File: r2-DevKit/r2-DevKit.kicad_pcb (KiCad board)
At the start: 4 copper layers, 92.3 x 67.1 mm, 33 parts, among them CON1 USB-MICRO-B, J1 CONN_01X05, J10 Battery SW, J11 OPTS, J2 CONN_01X08, J3 CONN_01X14, J4 CONN_01X02, J5 CONN_01X08, J6 CONN_01X14, J7 Li-Po, J8 JTAG, J9 CONN_02X15, P1 Compute Socket, P2 Sensor Socket, P3 CONN_01X01, P4 CONN_01X01, SW3 Pin_0, SW4 CHIP_PU, U1 EMIF02-USB03F2

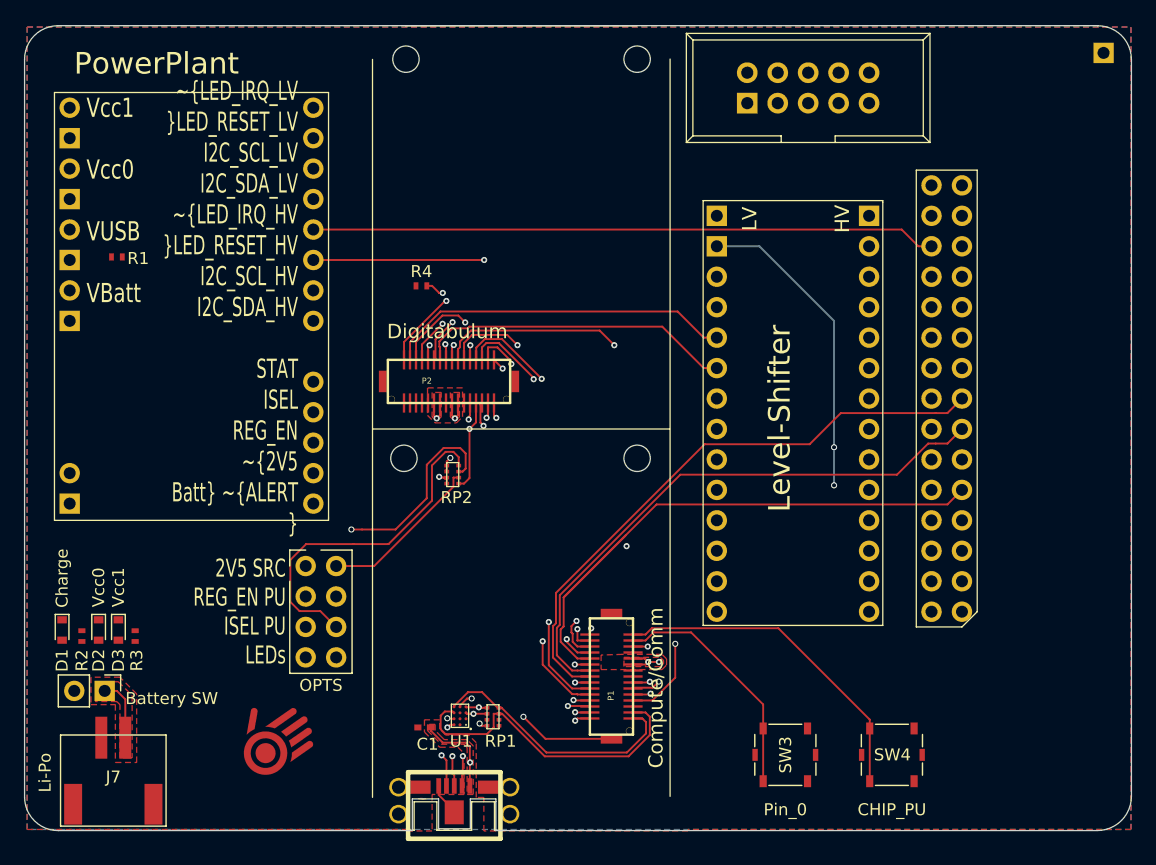
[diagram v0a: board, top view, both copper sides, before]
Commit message: Fixed some bugs in the Dev Harness.
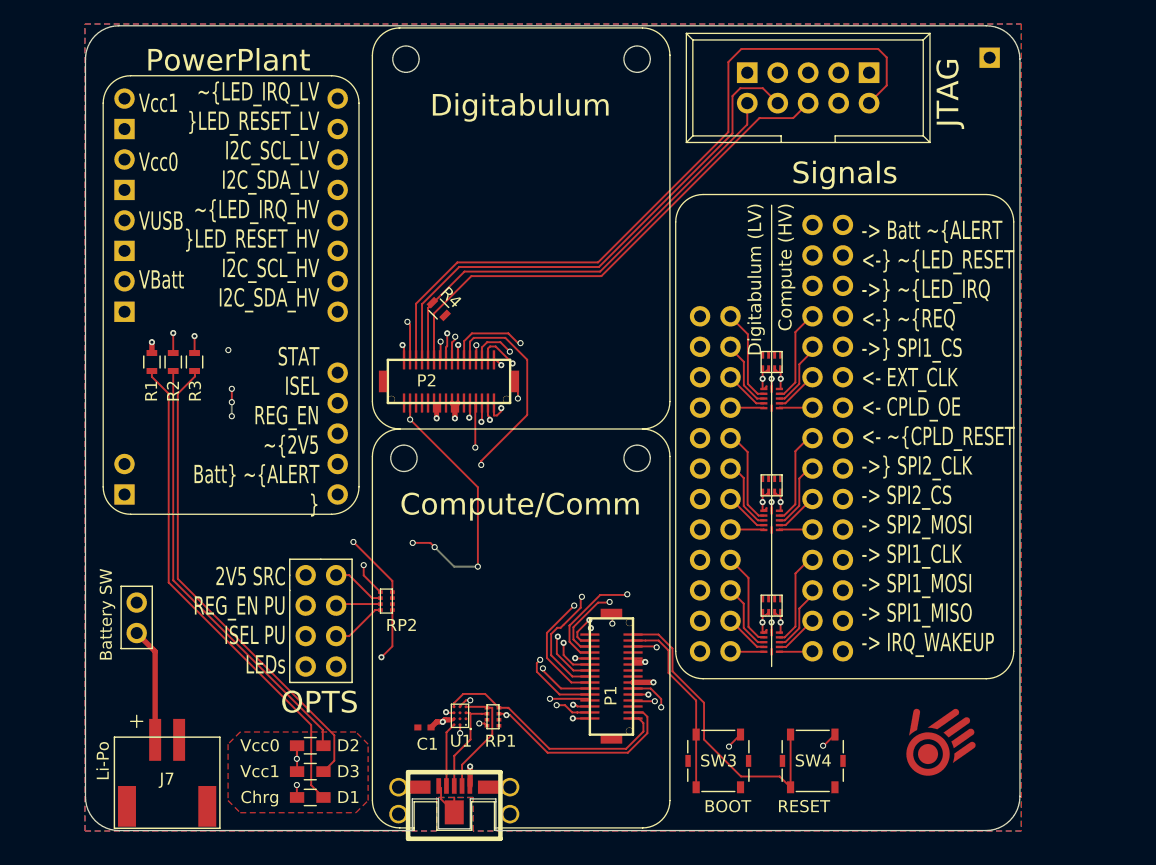
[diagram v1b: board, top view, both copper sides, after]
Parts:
- removed J6: CONN_01X14, Pin_Headers:Pin_Header_Straight_1x14_Pitch2.54mm
- added CARY1: 100nF, r2Parts:CapArray_CKCL44, F.Cu at (78.9, 56.3)
- added CARY2: 100nF, r2Parts:CapArray_CKCL44, F.Cu at (78.9, 66.3)
- added CARY3: 100nF, r2Parts:CapArray_CKCL44, F.Cu at (78.9, 46.0)
- added U2: LSF0204x, r2Parts:R-PUQFN-N12, F.Cu at (78.9, 69.3)
- added U3: LSF0204x, r2Parts:R-PUQFN-N12, F.Cu at (78.9, 59.2)
- added U4: LSF0204x, r2Parts:R-PUQFN-N12, F.Cu at (78.9, 49.0)
- D1: value Charge -> Chrg; footprint Diodes_SMD:D_0603 -> Resistors_SMD:R_0603_HandSoldering
- D2, D3: footprint Diodes_SMD:D_0603 -> Resistors_SMD:R_0603_HandSoldering
- J3: value CONN_01X14 -> Conn_02x12_Odd_Even; footprint Pin_Headers:Pin_Header_Straight_1x14_Pitch2.54mm -> Pin_Headers:Pin_Header_Straight_2x12_Pitch2.54mm
- R1, R4: footprint Resistors_SMD:R_0402_NoSilk -> Resistors_SMD:R_0603
- R2, R3: value 1k -> 680; footprint Resistors_SMD:R_0402_NoSilk -> Resistors_SMD:R_0603
- moved P3 55.3 mm to (92.5, 77.4)
- moved J3 36.3 mm to (75.4, 70.1), turned to 180 degrees
- moved D1 25.0 mm to (40.4, 82.3), turned to 0 degrees
- moved R2 24.1 mm to (29.0, 46.0)
- moved R3 23.4 mm to (30.7, 46.0)
- moved D2 20.1 mm to (40.4, 78.0), turned to 0 degrees
- moved D3 19.9 mm to (40.4, 80.1), turned to 0 degrees
- moved RP2 11.9 mm to (46.7, 65.9), turned to 0 degrees
- moved J9 10.5 mm to (84.8, 70.1)
- moved P4 9.51 mm to (97.1, 20.6)
- moved R1 9.24 mm to (27.2, 46.0), turned to 90 degrees
- moved SW4 6.62 mm to (82.3, 79.2)
- moved SW3 5.61 mm to (74.4, 79.2)
- moved J10 5.51 mm to (25.9, 68.6), turned to 180 degrees
- moved J4 4.64 mm to (24.9, 54.5)
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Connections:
- J3 pad 1: /VCC1 -> Net-(J3-Pad1)
- J3 pad 11: /SPI1_CLK -> Net-(J3-Pad11)
- J3 pad 12: /SPI1_MOSI -> /SPI2_CS
- J3 pad 13: /SPI1_MISO -> Net-(J3-Pad13)
- J3 pad 14: /IRQ_WAKEUP -> /SPI2_CLK
- J3 pad 2: GND -> /IRQ_WAKEUP
- J3 pad 3: /~REQ -> Net-(J3-Pad3)
- J3 pad 4: /SPI1_CS_0 -> /SPI1_MISO
- J3 pad 5: /CPLD_EXT_CLK -> Net-(J3-Pad5)
- J3 pad 6: /CPLD_OE -> /SPI1_MOSI
- J3 pad 7: /~CPLD_RESET -> Net-(J3-Pad7)
- J3 pad 8: /SPI2_CLK -> /SPI1_CLK
- J3 pad 9: /SPI2_CS -> Net-(J3-Pad9)
- J7 pad 1: GND -> Net-(J10-Pad1)
- J7 pad 2: Net-(J10-Pad1) -> GND
- J7 pad N0: (no net) -> GND
- J7 pad N1: (no net) -> GND
- J8 pad 6: (no net) -> Net-(J8-Pad6)
- J8 pad 7: (no net) -> Net-(J8-Pad7)
- J8 pad 8: (no net) -> Net-(J8-Pad8)
- P2 pad 11: (no net) -> Net-(P2-Pad11)
- P2 pad 5: (no net) -> Net-(P2-Pad5)
- P2 pad 8: (no net) -> Net-(P2-Pad8)
- P2 pad N0: (no net) -> GND
- P2 pad N1: (no net) -> GND
- U1 pad B1: (no net) -> Net-(U1-PadB1)
- U1 pad B2: (no net) -> Net-(U1-PadB2)
- U1 pad C2: (no net) -> Net-(U1-PadC2)
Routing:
- net /VCC0: track 34.6 -> 134.3 mm, vias 3 -> 6
- net /VCC1: track 135.4 -> 177.0 mm, vias 2 -> 6
- net Net-(D1-Pad2): track 0.00 -> 41.5 mm
- net Net-(D3-Pad2): track 0.00 -> 39.8 mm
- net Net-(D2-Pad2): track 0.00 -> 36.4 mm
- net Net-(J11-Pad6): track 28.6 -> 4.60 mm
- net Net-(J9-Pad9): track 51.0 -> 29.6 mm, vias 0 -> 1
- net Net-(J11-Pad4): track 22.4 -> 3.75 mm, vias 1 -> 0
- net Net-(J9-Pad11): track 50.0 -> 32.3 mm
- net /~LED_INT: track 41.1 -> 58.5 mm, vias 1 -> 2
- net /VCCUSB: track 110.5 -> 94.1 mm, vias 3 -> 4
- net /~LED_RESET_HV: track 53.1 -> 39.8 mm, vias 1 -> 0
- net /TDI: track 48.0 -> 60.9 mm, vias 1 -> 0
- net GND: track 38.9 -> 51.3 mm, vias 5 -> 14
- net Net-(J9-Pad13): track 47.7 -> 35.4 mm, vias 0 -> 1
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- added copper zone on Inner1.Cu, net GND
- added copper zone on Inner2.Cu, net GND
- removed copper zone on F.Cu, net /VCC0
- removed copper zone on F.Cu, net /VCC1
- removed copper zone on F.Cu, net /VCCUSB
- removed copper zone on Inner2.Cu, net /VCCUSB
- removed copper zone on F.Cu, net /Vbatt
- removed copper zone on Inner2.Cu, net /Vbatt
- removed copper zone on Inner2.Cu, net /Vlipo
- removed copper zone on F.Cu, net Net-(J10-Pad1)
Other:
- board size 92.3 x 67.1 mm -> 77.9 x 67.1 mm
- net class High-Current: trace_width 0.16 -> 0.45
- board text added: "-> Batt ~ALERT <- ~LED_RESET -> ~LED_IRQ <- ~REQ -> SPI1_CS <- EXT_CLK <- CPLD_OE <- ~CPLD_RESET -> SPI2_CLK -> SPI2_CS -> SPI2_MOSI -> SPI1_CLK -> SPI1_MOSI -> SPI1_MISO -> IRQ_WAKEUP"
- board text added: "All level-shifters are bi-directional LED PMIC signals are level-shifted alongside i2c on the PowerPlant board Battery alert signal does not require level-shifting"
- board text added: "BOOT RESET"
- board text added: "CPLD_GPIO REG_EN ISEL"
- board text added: "Compute"
- board text added: "Compute (HV)"
- board text added: "Dextral"
- board text added: "Digitabulum (LV)"
- board text added: "Digitabulum Dev Harness 2018-02-23 manuvr.io"
- board text added: "Distal"
- board text added: "Level Shift"
- board text added: "MAGNETOMETER KEEPOUT ZONE No copper on any layers Use only plastic retention hardware"
- board text added: "Signals"
- board text added: "Vcc1 Vcc0"
- board text added: "X"
- board text added: "Y"
- board text added: "Z"
- board text removed: "Batt ~ALERT ~LED_RESET ~LED_IRQ ~REQ SPI1_CS EXT_CLK CPLD_OE ~CPLD_RESET SPI2_CLK SPI2_CS SPI2_MOSI SPI1_CLK SPI1_MOSI SPI1_MISO IRQ_WAKEUP"
- board text removed: "Digitabulum Dev Harness 2017-10-05 manuvr.io"
- board text removed: "LV HV"
- board text removed: "Level-Shifter"
